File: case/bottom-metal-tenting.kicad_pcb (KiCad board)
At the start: 2 copper layers, 148 x 99.1 mm, 9 parts

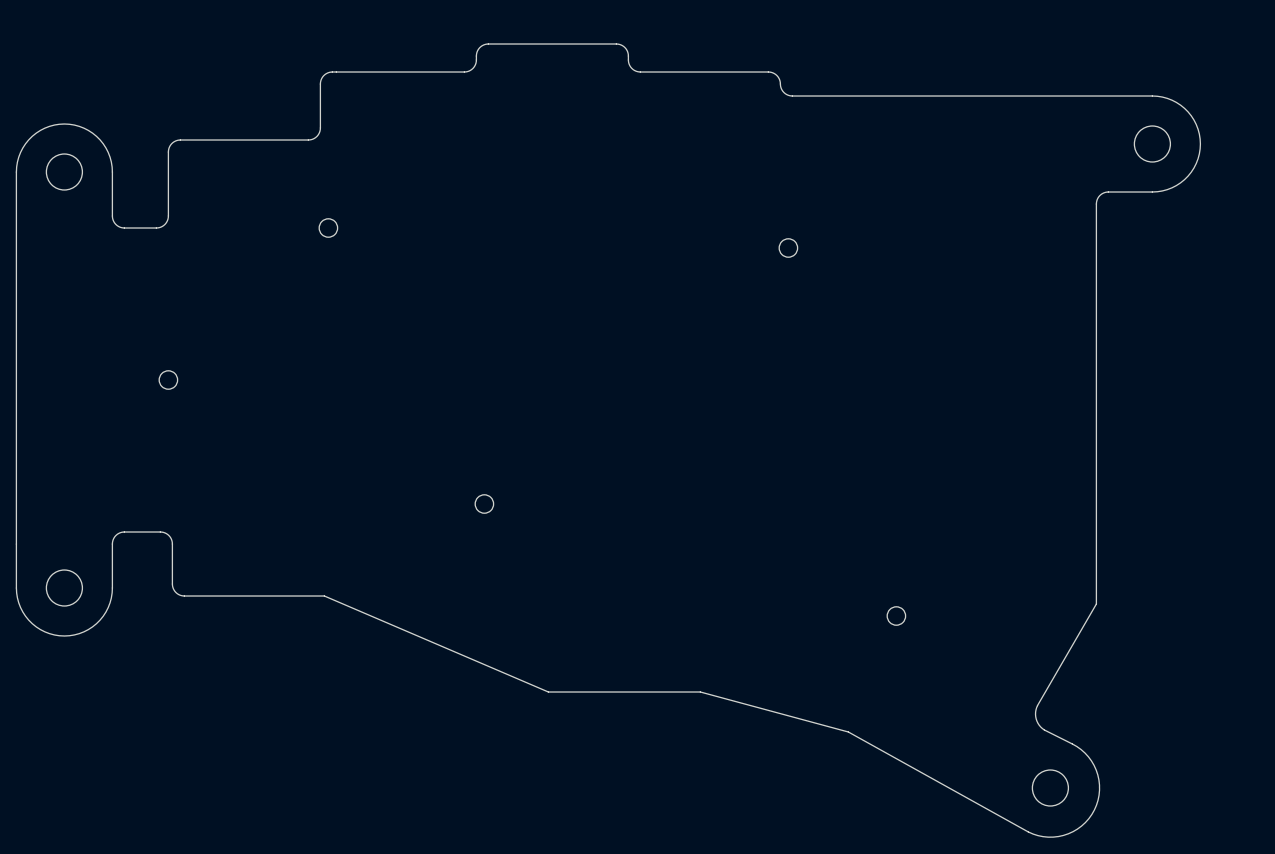
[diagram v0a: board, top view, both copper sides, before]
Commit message: update case files
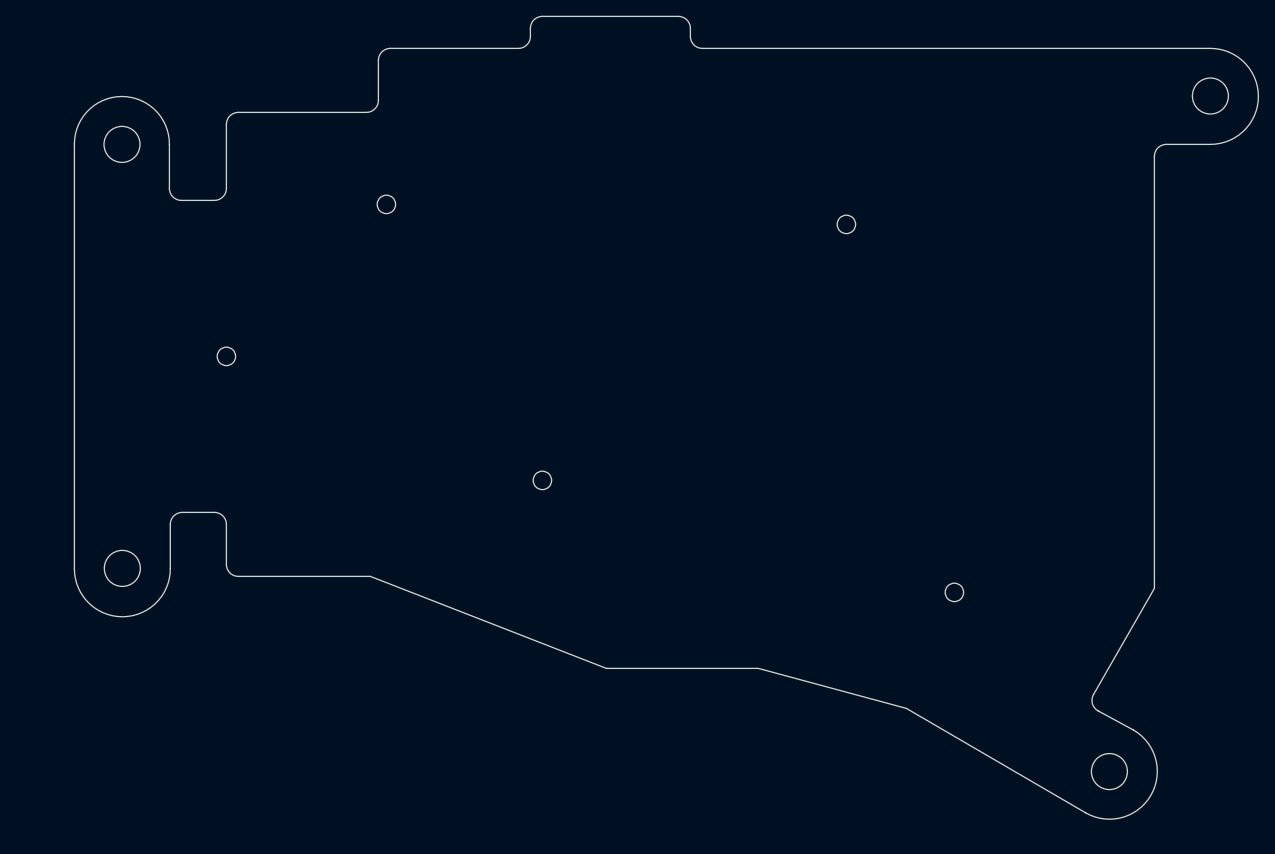
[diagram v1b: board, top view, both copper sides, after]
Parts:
- removed the REF** at (197.8, 144.5)
- removed the REF** at (74.5, 67.5)
- removed the REF** at (74.5, 119.5)
- removed the REF** at (210.5, 64.0)
- added REF**: MountingHole_4.5mm, MountingHole:MountingHole_4.5mm, F.Cu at (217.7, 58.0)
- added REF**: MountingHole_4.5mm, MountingHole:MountingHole_4.5mm, F.Cu at (205.1, 142.4)
- added REF**: MountingHole_4.5mm, MountingHole:MountingHole_4.5mm, F.Cu at (81.7, 64.0)
- added REF**: MountingHole_4.5mm, MountingHole:MountingHole_4.5mm, F.Cu at (81.7, 117.0)
- moved H1 7.83 mm to (114.8, 71.5)
- moved H2 7.83 mm to (185.8, 120.0)
- moved H3 7.83 mm to (94.8, 90.5)
- moved H4 7.83 mm to (134.2, 106.0)
- moved H5 7.83 mm to (172.2, 74.0)
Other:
- board size 148 x 99.1 mm -> 148 x 100.4 mm
